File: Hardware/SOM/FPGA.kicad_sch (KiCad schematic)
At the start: 77 parts, among them U1 LFE5UM5G-85F

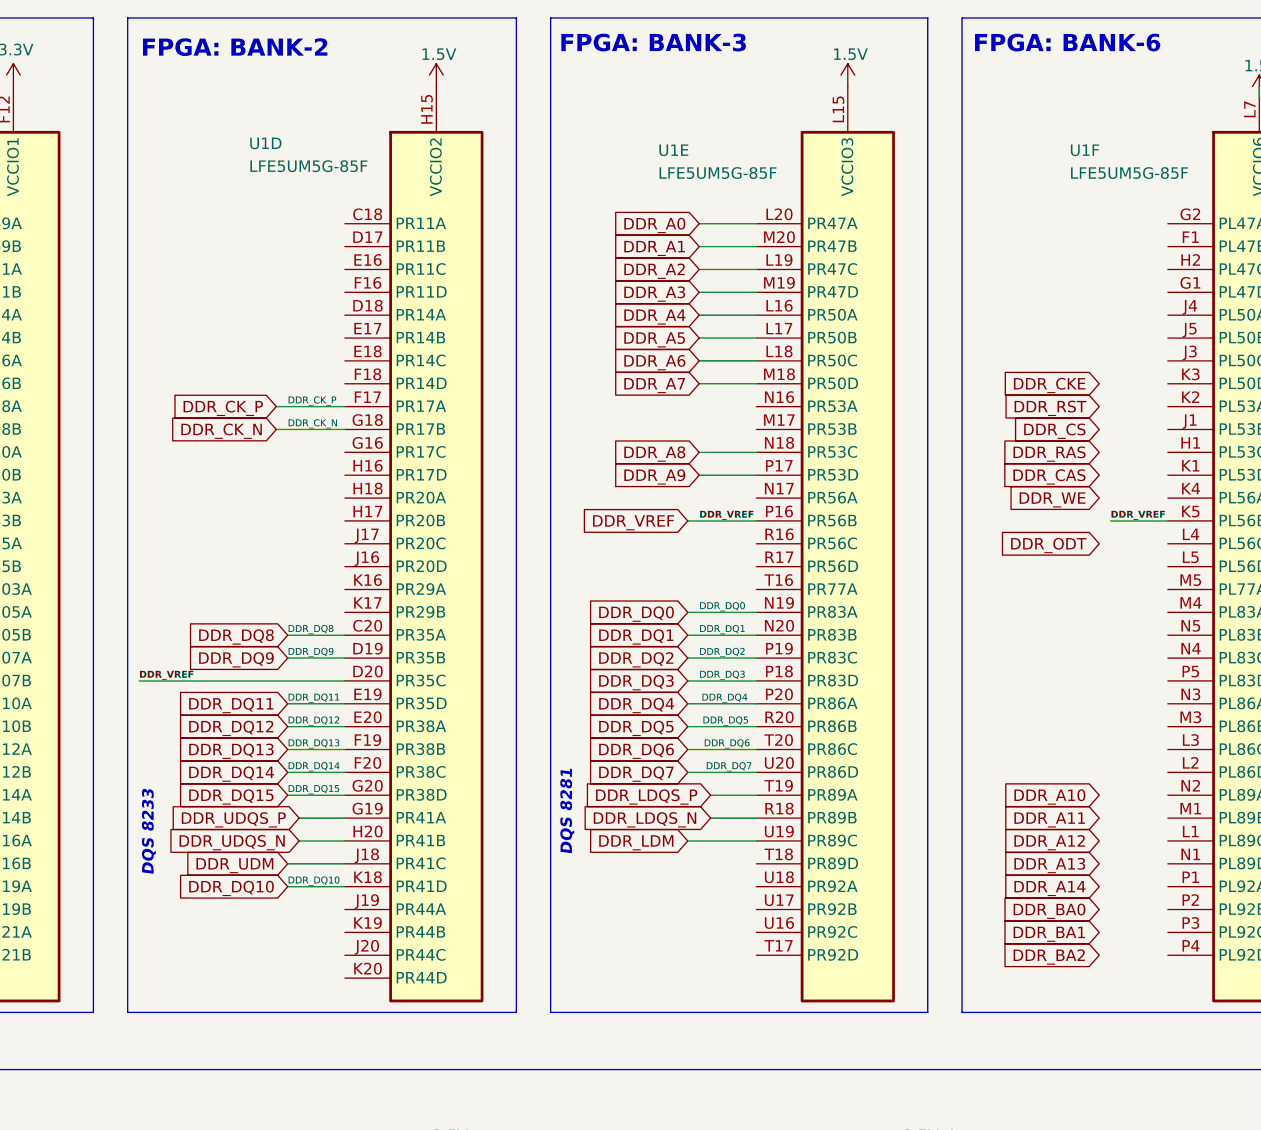
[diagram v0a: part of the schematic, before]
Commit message: DDR reconnect
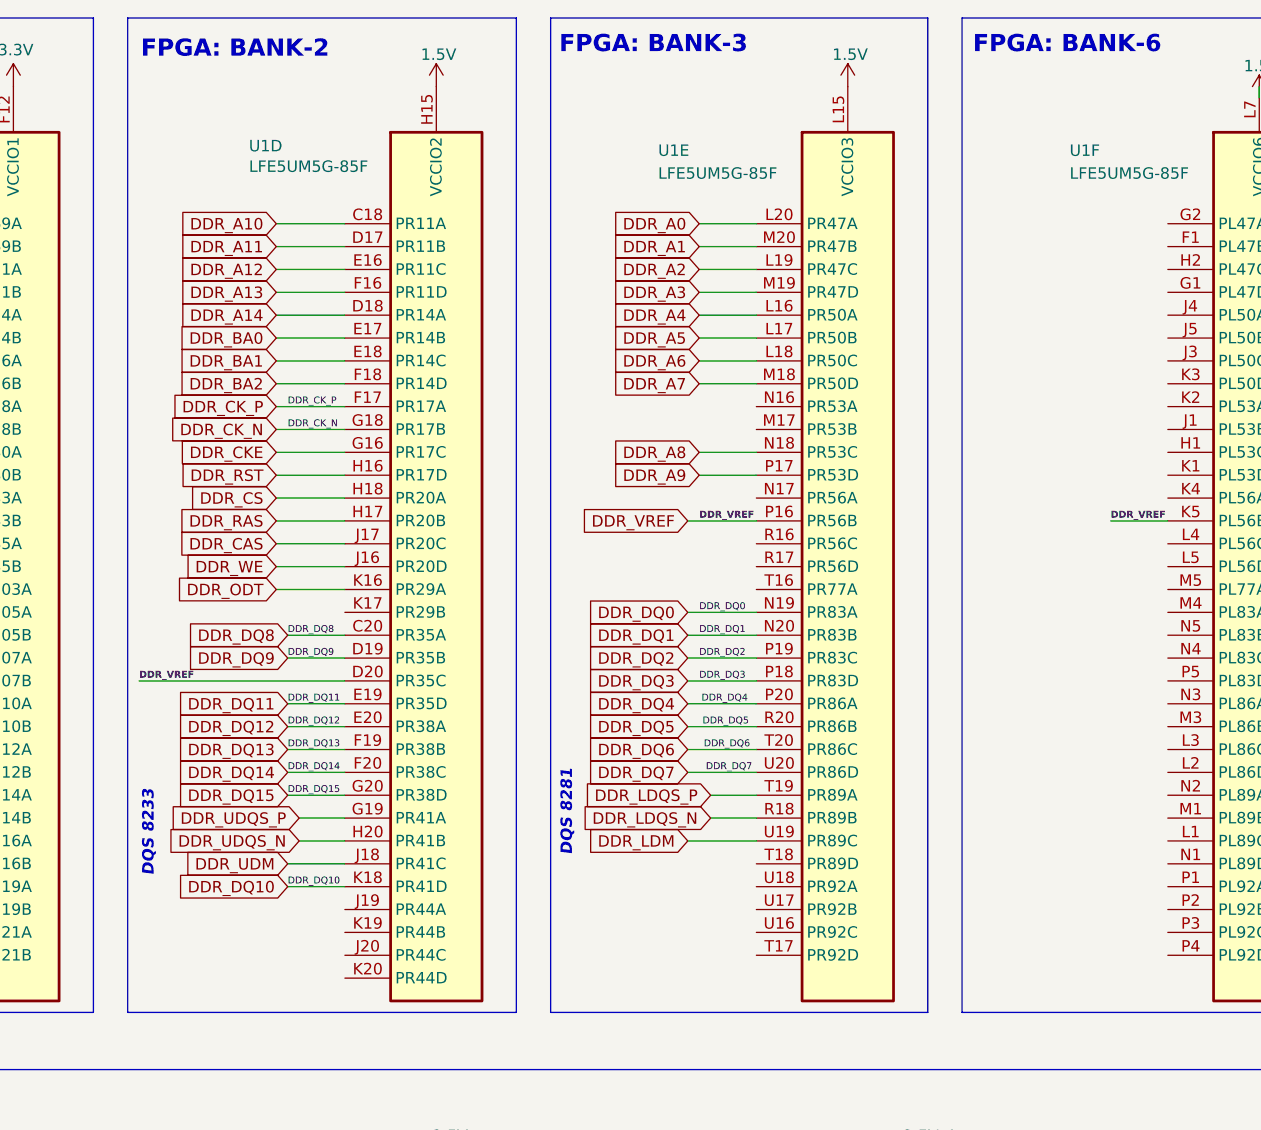
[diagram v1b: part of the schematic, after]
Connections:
- net DDR_A10: now also U1.C18 (PR11A)
- net DDR_A11: now also U1.D17 (PR11B)
- net DDR_A12: now also U1.E16 (PR11C)
- net DDR_A13: now also U1.F16 (PR11D)
- net DDR_A14: now also U1.D18 (PR14A)
- net DDR_BA0: now also U1.E17 (PR14B)
- net DDR_BA1: now also U1.E18 (PR14C)
- net DDR_BA2: now also U1.F18 (PR14D)
- net DDR_CAS: now also U1.J17 (PR20C)
- net DDR_CKE: now also U1.G16 (PR17C)
- net DDR_CS: now also U1.H18 (PR20A)
- net DDR_ODT: now also U1.K16 (PR29A)
- net DDR_RAS: now also U1.H17 (PR20B)
- net DDR_RST: now also U1.H16 (PR17D)
- net DDR_WE: now also U1.J16 (PR20D)
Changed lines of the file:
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@@
 	(wire
 		(pts
+			(xy 127 48.26) (xy 134.62 48.26)
+		)
+		(stroke
+			(width 0)
+			(type default)
+		)
+	)
+	(wire
+		(pts
 			(xy 165.1 179.07) (xy 157.48 179.07)
 		)
@@
 	(wire
 		(pts
+			(xy 127 73.66) (xy 134.62 73.66)
+		)
+		(stroke
+			(width 0)
+			(type default)
+		)
+	)
+	(wire
+		(pts
 			(xy 134.62 238.76) (xy 135.89 238.76)
 		)
@@
 	(wire
 		(pts
+			(xy 127 83.82) (xy 134.62 83.82)
+		)
+		(stroke
+			(width 0)
+			(type default)
+		)
+	)
+	(wire
+		(pts
 			(xy 195.58 191.77) (xy 207.01 191.77)
 		)
@@
 	(wire
 		(pts
+			(xy 127 53.34) (xy 134.62 53.34)
+		)
+		(stroke
+			(width 0)
+			(type default)
+		)
+	)
+	(wire
+		(pts
 			(xy 219.71 76.2) (xy 226.06 76.2)
 		)
@@
 	(wire
 		(pts
+			(xy 127 71.12) (xy 134.62 71.12)
+		)
+		(stroke
+			(width 0)
+			(type default)
+		)
+	)
+	(wire
+		(pts
 			(xy 173.99 43.18) (xy 180.34 43.18)
 		)
@@
 	(wire
 		(pts
+			(xy 127 81.28) (xy 134.62 81.28)
+		)
+		(stroke
+			(width 0)
+			(type default)
+		)
+	)
+	(wire
+		(pts
 			(xy 34.29 191.77) (xy 45.72 191.77)
 		)
@@
 	(wire
 		(pts
+			(xy 127 43.18) (xy 134.62 43.18)
+		)
+		(stroke
+			(width 0)
+			(type default)
+		)
+	)
+	(wire
+		(pts
 			(xy 184.15 208.28) (xy 185.42 208.28)
 		)
@@
 	(wire
 		(pts
+			(xy 127 45.72) (xy 134.62 45.72)
+		)
+		(stroke
+			(width 0)
+			(type default)
+		)
+	)
+	(wire
+		(pts
 			(xy 234.95 162.56) (xy 246.38 162.56)
 		)
@@
 	(wire
 		(pts
+			(xy 127 78.74) (xy 134.62 78.74)
+		)
+		(stroke
+			(width 0)
+			(type default)
+		)
+	)
+	(wire
+		(pts
 			(xy 63.5 151.13) (xy 71.12 151.13)
 		)
@@
 	(wire
 		(pts
+			(xy 127 76.2) (xy 134.62 76.2)
+		)
+		(stroke
+			(width 0)
+			(type default)
+		)
+	)
+	(wire
+		(pts
 			(xy 34.29 250.19) (xy 45.72 250.19)
 		)
@@
 	(wire
 		(pts
+			(xy 127 60.96) (xy 134.62 60.96)
+		)
+		(stroke
+			(width 0)
+			(type default)
+		)
+	)
+	(wire
+		(pts
 			(xy 165.1 208.28) (xy 157.48 208.28)
 		)
@@
 	(wire
 		(pts
+			(xy 127 50.8) (xy 134.62 50.8)
+		)
+		(stroke
+			(width 0)
+			(type default)
+		)
+	)
+	(wire
+		(pts
 			(xy 314.96 73.66) (xy 317.5 73.66)
 		)
@@
 	(wire
 		(pts
+			(xy 127 68.58) (xy 134.62 68.58)
+		)
+		(stroke
+			(width 0)
+			(type default)
+		)
+	)
+	(wire
+		(pts
+			(xy 127 58.42) (xy 134.62 58.42)
+		)
+		(stroke
+			(width 0)
+			(type default)
+		)
+	)
+	(wire
+		(pts
 			(xy 241.3 223.52) (xy 241.3 233.68)
 		)
@@
 	(wire
 		(pts
+			(xy 127 55.88) (xy 134.62 55.88)
+		)
+		(stroke
+			(width 0)
+			(type default)
+		)
+	)
+	(wire
+		(pts
 			(xy 165.1 236.22) (xy 165.1 238.76)
 		)
@@
 	(global_label "DDR_A13"
 		(shape input)
-		(at 218.44 114.3 180)
+		(at 127 50.8 180)
 		(fields_autoplaced yes)
 		(effects
@@
 		)
 		(property "Intersheetrefs" "${INTERSHEET_REFS}"
-			(at 207.1696 114.3 0)
+			(at 115.7296 50.8 0)
 			(effects
 				(font
@@
 	(global_label "DDR_WE"
 		(shape input)
-		(at 218.44 73.66 180)
+		(at 127 81.28 180)
 		(fields_autoplaced yes)
 		(effects
@@
 		)
 		(property "Intersheetrefs" "${INTERSHEET_REFS}"
-			(at 208.0768 73.66 0)
+			(at 116.6368 81.28 0)
 			(effects
 				(font
@@
 	(global_label "DDR_A11"
 		(shape input)
-		(at 218.44 109.22 180)
+		(at 127 45.72 180)
 		(fields_autoplaced yes)
 		(effects
@@
 		)
 		(property "Intersheetrefs" "${INTERSHEET_REFS}"
-			(at 207.1696 109.22 0)
+			(at 115.7296 45.72 0)
 			(effects
 				(font
@@
 	(global_label "DDR_BA2"
 		(shape input)
-		(at 218.44 124.46 180)
+		(at 127 60.96 180)
 		(fields_autoplaced yes)
 		(effects
@@
 		)
 		(property "Intersheetrefs" "${INTERSHEET_REFS}"
-			(at 207.1091 124.46 0)
+			(at 115.6691 60.96 0)
 			(effects
 				(font
@@
 	(global_label "DDR_CAS"
 		(shape input)
-		(at 218.44 71.12 180)
+		(at 127 78.74 180)
 		(fields_autoplaced yes)
 		(effects
@@
 		)
 		(property "Intersheetrefs" "${INTERSHEET_REFS}"
-			(at 207.1091 71.12 0)
+			(at 115.6691 78.74 0)
 			(effects
 				(font
@@
 	(global_label "DDR_A10"
 		(shape input)
-		(at 218.44 106.68 180)
+		(at 127 43.18 180)
 		(fields_autoplaced yes)
 		(effects
@@
 		)
 		(property "Intersheetrefs" "${INTERSHEET_REFS}"
-			(at 207.1696 106.68 0)
+			(at 115.7296 43.18 0)
 			(effects
 				(font
@@
 	(global_label "DDR_A12"
 		(shape input)
-		(at 218.44 111.76 180)
+		(at 127 48.26 180)
 		(fields_autoplaced yes)
 		(effects
@@
 		)
 		(property "Intersheetrefs" "${INTERSHEET_REFS}"
-			(at 207.1696 111.76 0)
+			(at 115.7296 48.26 0)
 			(effects
 				(font
@@
 	(global_label "DDR_RAS"
 		(shape input)
-		(at 218.44 68.58 180)
+		(at 127 76.2 180)
 		(fields_autoplaced yes)
 		(effects
@@
 		)
 		(property "Intersheetrefs" "${INTERSHEET_REFS}"
-			(at 207.1091 68.58 0)
+			(at 115.6691 76.2 0)
 			(effects
 				(font
@@
 	(global_label "DDR_RST"
 		(shape input)
-		(at 218.44 63.5 180)
+		(at 127 71.12 180)
 		(fields_autoplaced yes)
 		(effects
@@
 		)
 		(property "Intersheetrefs" "${INTERSHEET_REFS}"
-			(at 207.2301 63.5 0)
+			(at 115.7901 71.12 0)
 			(effects
 				(font
@@
 	(global_label "DDR_A14"
 		(shape input)
-		(at 218.44 116.84 180)
+		(at 127 53.34 180)
 		(fields_autoplaced yes)
 		(effects
@@
 		)
 		(property "Intersheetrefs" "${INTERSHEET_REFS}"
-			(at 207.1696 116.84 0)
+			(at 115.7296 53.34 0)
 			(effects
 				(font
@@
 	(global_label "DDR_BA0"
 		(shape input)
-		(at 218.44 119.38 180)
+		(at 127 55.88 180)
 		(fields_autoplaced yes)
 		(effects
@@
 		)
 		(property "Intersheetrefs" "${INTERSHEET_REFS}"
-			(at 207.1091 119.38 0)
+			(at 115.6691 55.88 0)
 			(effects
 				(font
@@
 	(global_label "DDR_ODT"
 		(shape input)
-		(at 218.44 78.74 180)
+		(at 127 83.82 180)
 		(fields_autoplaced yes)
 		(effects
@@
 		)
 		(property "Intersheetrefs" "${INTERSHEET_REFS}"
-			(at 207.1091 78.74 0)
+			(at 115.6691 83.82 0)
 			(effects
 				(font
@@
 	(global_label "DDR_BA1"
 		(shape input)
-		(at 218.44 121.92 180)
+		(at 127 58.42 180)
 		(fields_autoplaced yes)
 		(effects
@@
 		)
 		(property "Intersheetrefs" "${INTERSHEET_REFS}"
-			(at 207.1091 121.92 0)
+			(at 115.6691 58.42 0)
 			(effects
 				(font
@@
 	(global_label "DDR_CS"
 		(shape input)
-		(at 218.44 66.04 180)
+		(at 127 73.66 180)
 		(fields_autoplaced yes)
 		(effects
@@
 		)
 		(property "Intersheetrefs" "${INTERSHEET_REFS}"
-			(at 208.1977 66.04 0)
+			(at 116.7577 73.66 0)
 			(effects
 				(font
@@
 	(global_label "DDR_CKE"
 		(shape input)
-		(at 218.44 60.96 180)
+		(at 127 68.58 180)
 		(fields_autoplaced yes)
 		(effects
@@
 		)
 		(property "Intersheetrefs" "${INTERSHEET_REFS}"
-			(at 206.9882 60.96 0)
+			(at 115.5482 68.58 0)
 			(effects
 				(font
@@
 		(dnp no)
 		(property "Reference" "U1"
-			(at 123.952 34.29 0)
+			(at 123.952 34.544 0)
 			(effects
 				(font
